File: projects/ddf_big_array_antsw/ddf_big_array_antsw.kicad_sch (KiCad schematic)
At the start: 35 parts, among them J1 Conn_Coaxial, J2 Conn_Coaxial, J3 Conn_Coaxial, J4 Conn_Coaxial, J5 Conn_Coaxial, J6 RJ45_Shielded

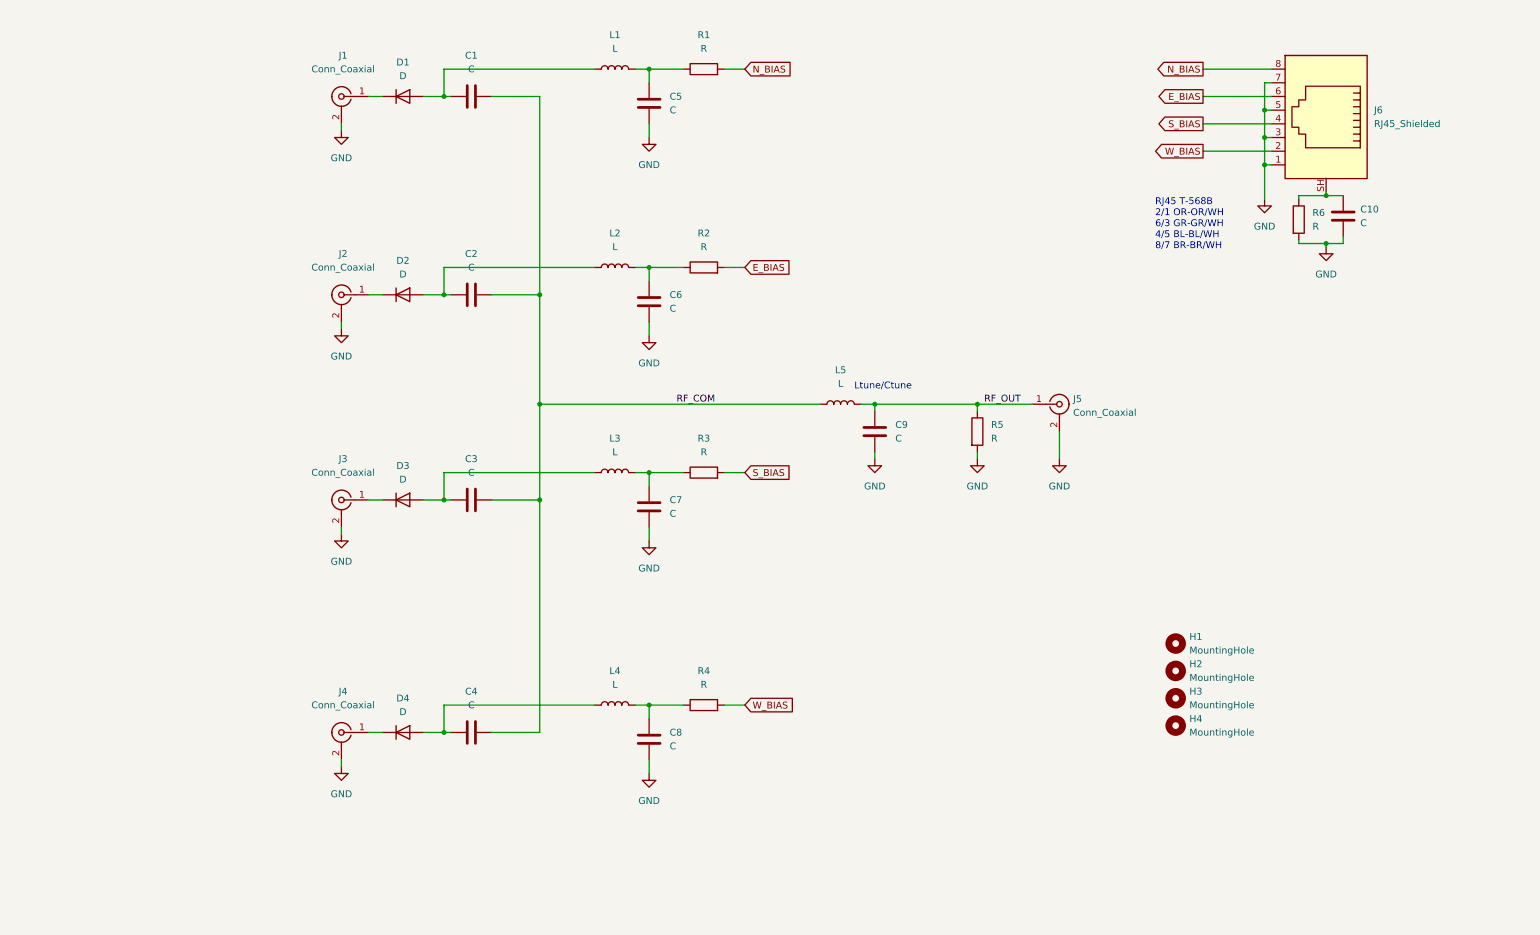
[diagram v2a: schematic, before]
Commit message: Closing on release quality.
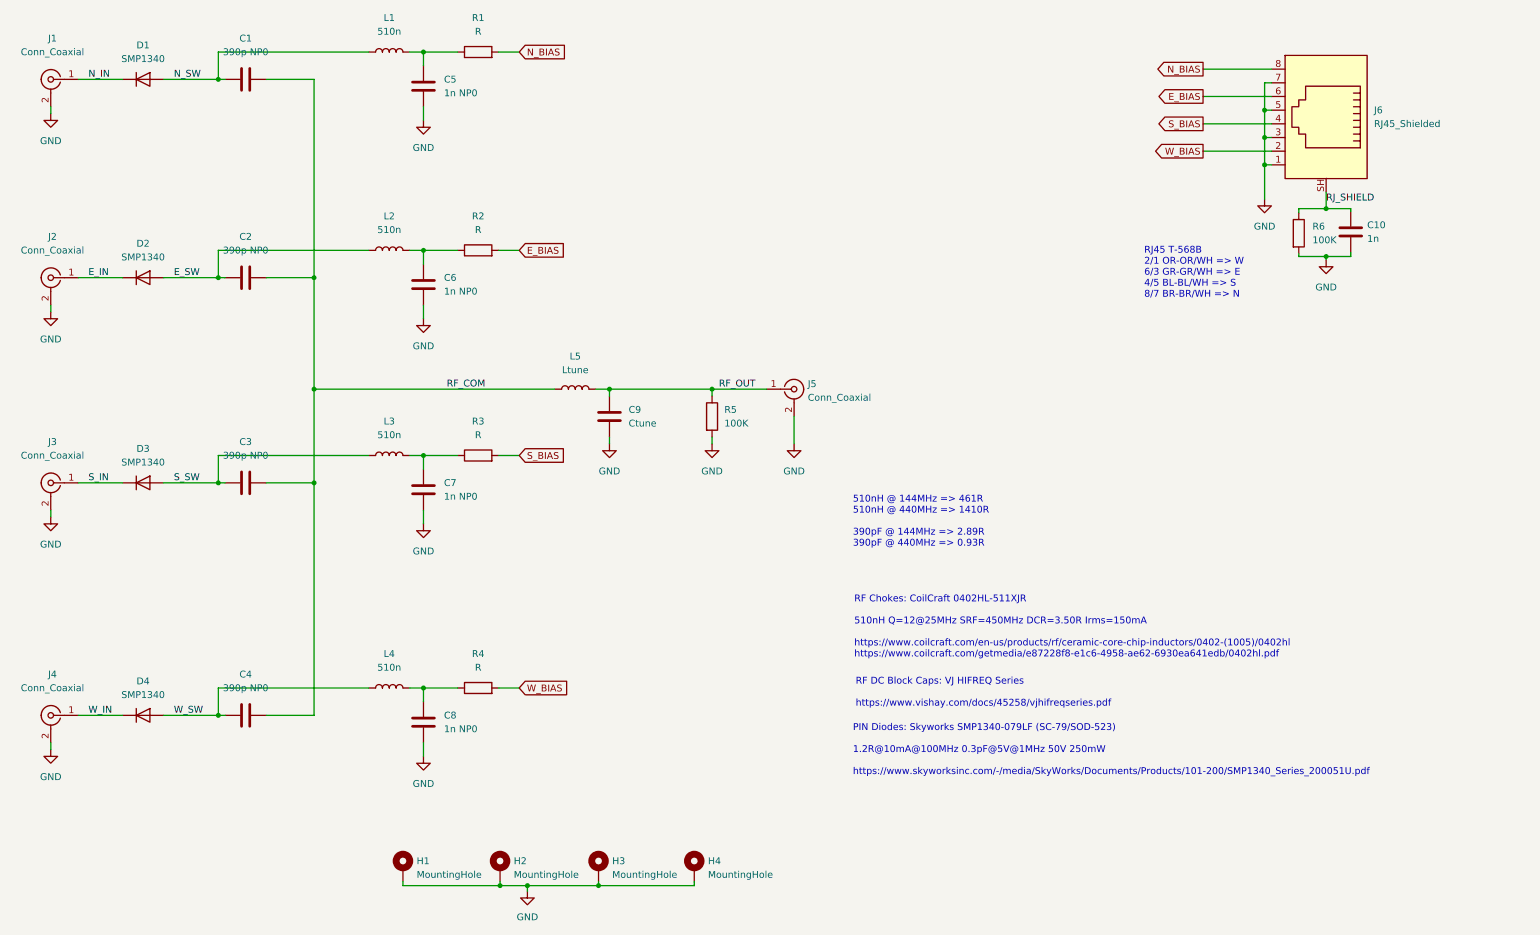
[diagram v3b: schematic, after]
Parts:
- C1, C2, C3, C4: value C -> 390p NP0; footprint Capacitor_SMD:C_0402_1005Metric_Pad0.74x0.62mm_HandSolder -> Capacitor_SMD:C_0603_1608Metric_Pad1.08x0.95mm_HandSolder
- C10: value C -> 1n
- C5, C6, C7, C8: value C -> 1n NP0
- C9: value C -> Ctune; footprint Capacitor_SMD:C_0603_1608Metric_Pad1.08x0.95mm_HandSolder -> Capacitor_SMD:C_0402_1005Metric_Pad0.74x0.62mm_HandSolder
- D1, D2, D3, D4: value D -> SMP1340
- H1, H2, H3, H4: footprint MountingHole:MountingHole_3.2mm_M3 -> MountingHole:MountingHole_3.2mm_M3_Pad_TopBottom; symbol Mechanical:MountingHole -> Mechanical:MountingHole_Pad
- J1, J2, J3, J4, J5: footprint Connector_Coaxial:SMA_Amphenol_132203-12_Horizontal -> ch:SMA_Molex_73251-2200_Horizontal
- L1, L2, L3, L4: value L -> 510n; footprint Inductor_SMD:L_0402_1005Metric_Pad0.77x0.64mm_HandSolder -> ch:Coilcraft-0402HL-hand-solder
- L5: value L -> Ltune
- R5, R6: value R -> 100K
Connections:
- net GND: now also H1.1, H2.1, H3.1, H4.1
- net S_SW: now reaches C3.1, D3.2 (A), L3.1
- net E_SW: now reaches C2.1, D2.2 (A), L2.1
- net W_SW: now reaches C4.1, D4.2 (A), L4.1
- net RJ_SHIELD: now reaches C10.1, J6.SH, R6.1
- net N_IN: now reaches D1.1 (K), J1.1 (In)
- net E_IN: now reaches D2.1 (K), J2.1 (In)
- net N_SW: now reaches C1.1, D1.2 (A), L1.1
- net S_IN: now reaches D3.1 (K), J3.1 (In)
- net W_IN: now reaches D4.1 (K), J4.1 (In)
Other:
- note added: "510nH @ 144MHz => 461R 510nH @ 440MHz => 1410R 390pF @ 144MHz => 2.89R 390pF @ 440MHz => 0.93R"
- note added: "PIN Diodes: Skyworks SMP1340-079LF (SC-79/SOD-523) 1.2R@10mA@100MHz 0.3pF@5V@1MHz 50V 250mW https://www.skyworksinc.com/-/media/SkyWorks/Documents/Products/101-200/SMP1340_Series_200051U.pdf"
- note added: "RF Chokes: CoilCraft 0402HL-511XJR 510nH Q=12@25MHz SRF=450MHz DCR=3.50R Irms=150mA https://www.coilcraft.com/en-us/products/rf/ceramic-core-chip-inductors/0402-(1005)/0402hl https://www.coilcraft.com/getmedia/e87228f8-e1c6-4958-ae62-6930ea641edb/0402hl.pdf"
- note added: "RF DC Block Caps: VJ HIFREQ Series https://www.vishay.com/docs/45258/vjhifreqseries.pdf"
- note added: "RJ45 T-568B 2/1 OR-OR/WH => W 6/3 GR-GR/WH => E 4/5 BL-BL/WH => S 8/7 BR-BR/WH => N"
- note removed: "Ltune/Ctune"
- note removed: "RJ45 T-568B 2/1 OR-OR/WH 6/3 GR-GR/WH 4/5 BL-BL/WH 8/7 BR-BR/WH"
- moved on the sheet: C1, C10, C2, C3, C4, C5, C6, C7, C8, C9, D1, D2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
